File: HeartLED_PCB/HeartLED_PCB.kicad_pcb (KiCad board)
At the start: 2 copper layers, 58.8 x 52.2 mm, 37 parts, among them U1 ICM7555IBAZ-T, U2 CD4017BM96, U3 TPS61222DCKR, U4 HX SS12F44G4

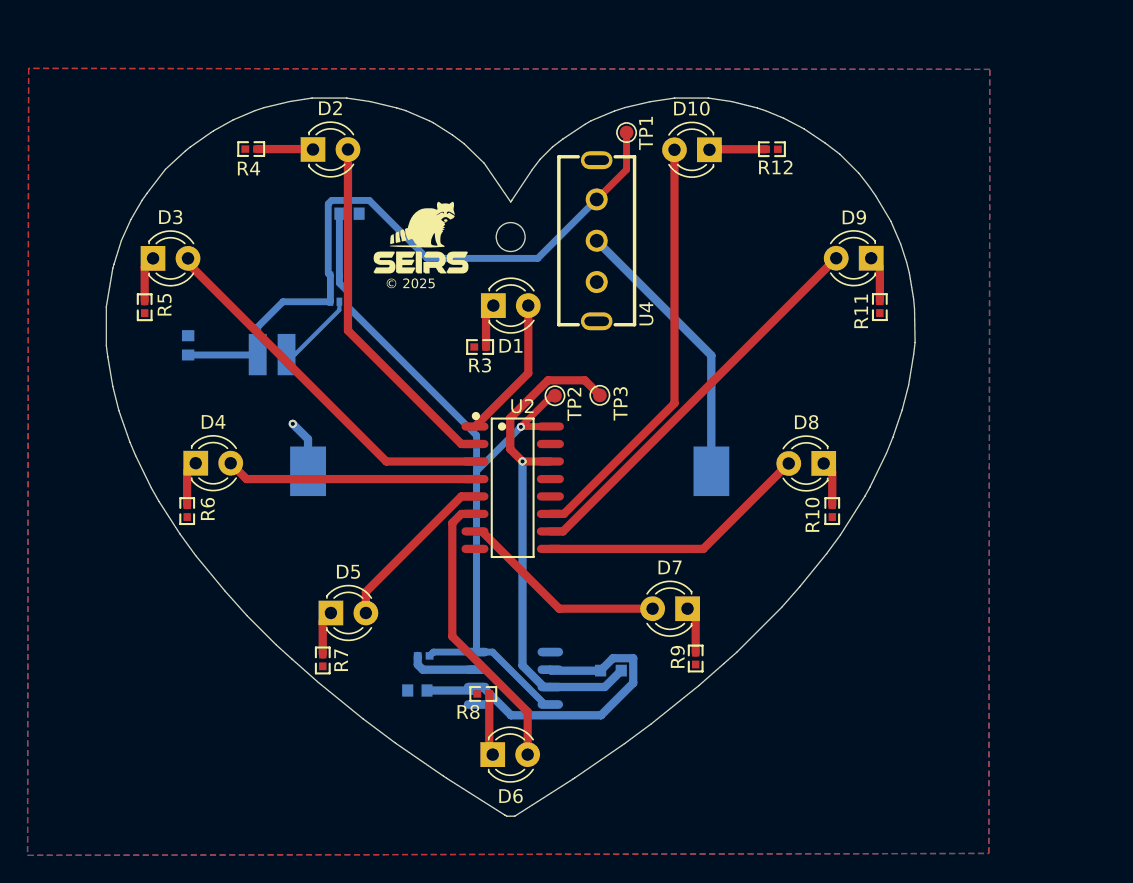
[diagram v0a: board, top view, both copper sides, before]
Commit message: Ready to route
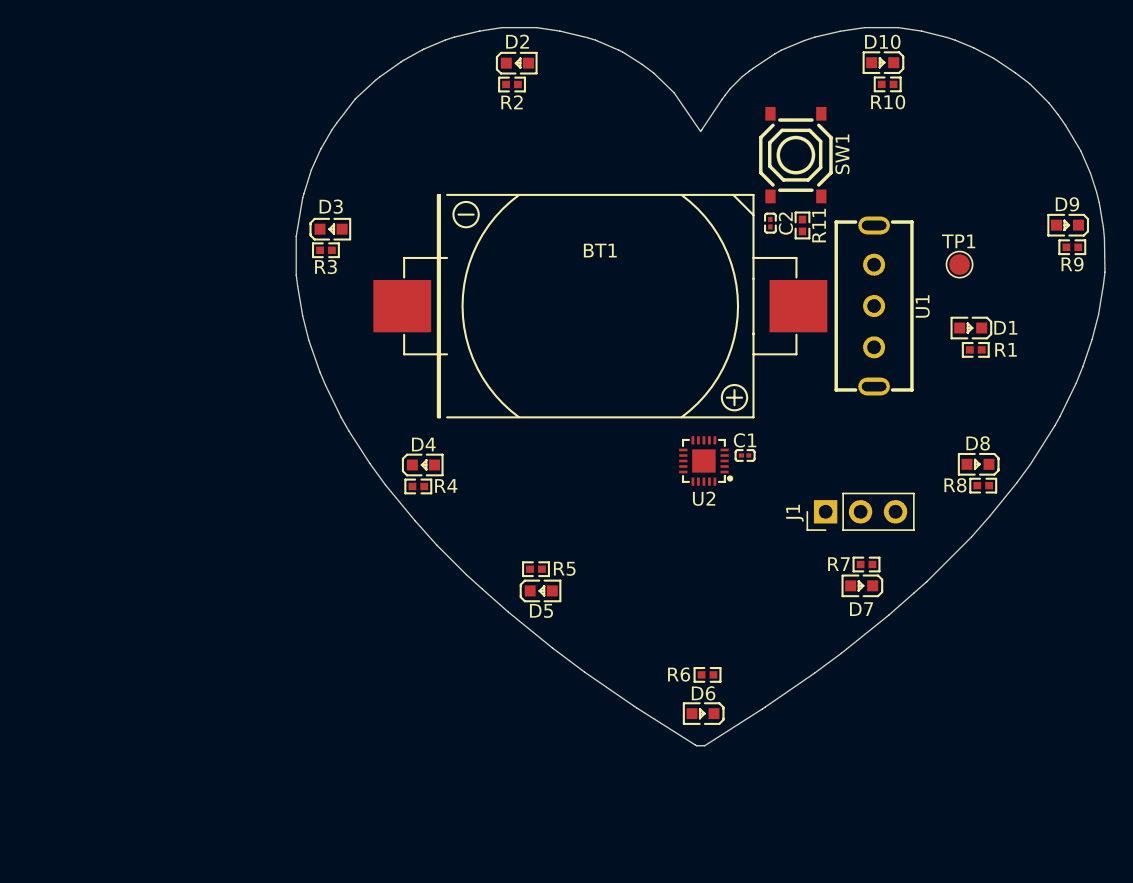
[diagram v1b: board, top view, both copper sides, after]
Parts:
- removed C3: 10uF, FOOTPRINTS:CL10A106MQ8NNNC
- removed G***: LOGO, FOOTPRINTS:seirslogo
- removed G***: LOGO, FOOTPRINTS:raccoonimage
- removed H1: MountingHole, MountingHole:MountingHole_2.1mm
- removed L1: 4.7uH, FOOTPRINTS:LQH3NPN4R7MMEL
- removed R12: 3.3k, FOOTPRINTS:0402WGJ0332TCE
- removed TP2, TP3: TestPoint, TestPoint:TestPoint_Pad_D1.0mm
- removed U3: TPS61222DCKR, FOOTPRINTS:TPS61222DCKR
- removed U4: HX SS12F44G4, FOOTPRINTS:HX SS12F44G4
- added J1: Conn_01x03, Connector_PinHeader_2.54mm:PinHeader_1x03_P2.54mm_Vertical, F.Cu at (152.9, 102.6)
- added SW1: TS-1187A-B-A-B, FOOTPRINTS:TS-1187A-B-A-B, F.Cu at (150.7, 76.7)
- BT1: value Battery_Cell -> CR2032-BS-6-1; footprint Battery:BatteryHolder_Keystone_1060_1x2032 -> FOOTPRINTS:CR2032-BS-6-1; moved to F.Cu
- C1: value 4.7uF -> 100nF; footprint FOOTPRINTS:CL10A475KP8NNNC -> FOOTPRINTS:0201X104K100CT; moved to F.Cu
- C2: value 10uF -> 100nF; footprint FOOTPRINTS:CL10A106MQ8NNNC -> FOOTPRINTS:0201X104K100CT; moved to F.Cu
- D1: footprint LED_THT:LED_D3.0mm -> FOOTPRINTS:F.0603.00026_P2-0603B1TS2-06T-001
- D10, D2, D3, D4, D5, D6, D7, D8, D9: footprint LED_THT:LED_D3.0mm -> FOOTPRINTS:F.0603.00139_P2-0603R1TS2-06T-002
- R1: value 100k -> 1k; footprint FOOTPRINTS:0603WAJ0104T5E -> FOOTPRINTS:0402WGJ0102TCE; moved to F.Cu
- R10, R11, R3, R4, R5, R6, R7, R8, R9: value 3.3k -> 1k; footprint FOOTPRINTS:0402WGJ0332TCE -> FOOTPRINTS:0402WGJ0102TCE
- R2: value 10k -> 1k; footprint FOOTPRINTS:0402WGJ0103TCE -> FOOTPRINTS:0402WGJ0102TCE; moved to F.Cu
- TP1: footprint TestPoint:TestPoint_Pad_D1.0mm -> TestPoint:TestPoint_Pad_D1.5mm
- U1: value ICM7555IBAZ-T -> HX SS12F44G4; footprint FOOTPRINTS:ICM7555IBAZ-T -> FOOTPRINTS:HX SS12F44G4; moved to F.Cu
- U2: value CD4017BM96 -> ATTINY816-MN_C617908; footprint FOOTPRINTS:CD4017BM96 -> FOOTPRINTS:ATTINY816-MN
- moved C2 43.2 mm to (148.9, 81.6), turned to -90 degrees
- moved R2 42.0 mm to (130.1, 71.5), turned to 180 degrees
- moved R9 40.5 mm to (170.8, 83.3), turned to 0 degrees
- moved R7 40.1 mm to (155.8, 106.4), turned to 0 degrees
- moved R6 39.6 mm to (144.3, 114.4), turned to 0 degrees
- moved R8 39.3 mm to (164.3, 100.7), turned to 0 degrees
- moved U1 37.7 mm to (156.4, 87.6), turned to 90 degrees
- moved R1 35.3 mm to (163.8, 90.8), turned to 0 degrees
- moved D1 34.7 mm to (163.4, 89.2), turned to 180 degrees
- moved R5 34.2 mm to (131.8, 106.7), turned to 180 degrees
- moved R10 31.3 mm to (157.4, 71.5), turned to 180 degrees
- moved C1 29.3 mm to (147.0, 98.5)
- moved R4 27.4 mm to (123.3, 100.7)
- moved TP1 26.0 mm to (162.6, 84.6), turned to 0 degrees
- moved D4 16.5 mm to (123.7, 99.2)
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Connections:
- C1 pad 1: Net-(U1-THRESHOLD) -> GND
- C1 pad 2: GND -> +3V0
- C2 pad 1: +3V -> PB4
- D1 pad 2: Net-(D1-A) -> +3V0
- D10 pad 2: Net-(D10-A) -> PA4
- D2 pad 2: Net-(D2-A) -> PB1
- D3 pad 2: Net-(D3-A) -> PB0
- D4 pad 2: Net-(D4-A) -> PC0
- D5 pad 2: Net-(D5-A) -> PC1
- D6 pad 2: Net-(D6-A) -> PC2
- D7 pad 2: Net-(D7-A) -> PC3
- D8 pad 2: Net-(D8-A) -> PA1
- D9 pad 2: Net-(D9-A) -> PA2
- R1 pad 1: ASTABLE_OUTPUT -> GND
- R1 pad 2: Net-(U1-THRESHOLD) -> Net-(D1-K)
- R10 pad 1: GND -> Net-(D10-K)
- R10 pad 2: Net-(D8-K) -> GND
- R11 pad 1: GND -> +3V0
- R11 pad 2: Net-(D9-K) -> PB4
- R2 pad 1: Net-(U1-DISCHARGE) -> GND
- R2 pad 2: +5V -> Net-(D2-K)
- R3 pad 1: Net-(D1-K) -> GND
- R3 pad 2: GND -> Net-(D3-K)
- R4 pad 1: Net-(D2-K) -> GND
- R4 pad 2: GND -> Net-(D4-K)
- R5 pad 1: Net-(D3-K) -> GND
- R5 pad 2: GND -> Net-(D5-K)
- R6 pad 1: Net-(D4-K) -> GND
- R6 pad 2: GND -> Net-(D6-K)
- R7 pad 2: Net-(D5-K) -> Net-(D7-K)
- R8 pad 1: Net-(D6-K) -> GND
- R8 pad 2: GND -> Net-(D8-K)
- R9 pad 1: Net-(D7-K) -> GND
- R9 pad 2: GND -> Net-(D9-K)
- TP1 pad 1: +3V -> +3V0
- U1 pad 1: GND -> unconnected-(U1-Pad1)
- U1 pad 2: Net-(U1-THRESHOLD) -> Net-(BT1-+)
- U1 pad 3: ASTABLE_OUTPUT -> +3V0
- U1 pad 4: +5V -> unconnected-(U1-Pad4)
- U1 pad 5: GND -> unconnected-(U1-Pad5)
- U2 pad 1: Net-(D1-A) -> PA2
- U2 pad 10: Net-(D9-A) -> PB4
- U2 pad 11: Net-(D10-A) -> unconnected-(U2-PB3/TOSC1-Pad11)
- U2 pad 13: GND -> PB1
- U2 pad 14: ASTABLE_OUTPUT -> PB0
- U2 pad 15: unconnected-(U2-RESET-Pad15) -> PC0
- U2 pad 16: +5V -> PC1
- U2 pad 2: Net-(D2-A) -> unconnected-(U2-EXTCLK/PA3-Pad2)
- U2 pad 3: Net-(D3-A) -> GND
- U2 pad 4: Net-(D4-A) -> +3V0
- U2 pad 5: Net-(D5-A) -> PA4
- U2 pad 6: Net-(D6-A) -> PA5
- U2 pad 7: Net-(D7-A) -> unconnected-(U2-PA6-Pad7)
- U2 pad 8: GND -> unconnected-(U2-PA7-Pad8)
- U2 pad 9: Net-(D8-A) -> unconnected-(U2-PB5-Pad9)
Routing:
- net +5V: track 69.5 -> 0.00 mm, vias 1 -> 0
- net +3V: track 49.1 -> 0.00 mm
- net ASTABLE_OUTPUT: track 36.8 -> 0.00 mm, vias 1 -> 0
- net Net-(D10-A): track 30.8 -> 0.00 mm
- net Net-(D9-A): track 29.0 -> 0.00 mm
- net Net-(D3-A): track 27.3 -> 0.00 mm
- net Net-(D2-A): track 25.8 -> 0.00 mm
- net Net-(U1-THRESHOLD): track 25.1 -> 0.00 mm
- net Net-(D6-A): track 21.0 -> 0.00 mm
- net Net-(BT1-+): track 20.2 -> 0.00 mm
- net Net-(D8-A): track 19.9 -> 0.00 mm
- net Net-(D4-A): track 18.2 -> 0.00 mm
- net Net-(D7-A): track 14.7 -> 0.00 mm
- net Net-(D5-A): track 12.3 -> 0.00 mm
- net Net-(D1-A): track 10.4 -> 0.00 mm
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- removed copper zone on B.Cu, net GND
- removed copper zone on F.Cu, net GND
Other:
- board text removed: "Happy Valentine's Day ( ˘ ³˘)♥"
- board text removed: "github.com/ fectec/ HeartLED"
- board text removed: "v1.0.0"
- board text removed: "© 2025"
